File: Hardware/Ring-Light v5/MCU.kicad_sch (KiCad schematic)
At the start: 55 parts, among them J2 1017457000B11LF, J3 U.FL-R-SMT-1_80, J4 2002112100010C4LF, U37 CP2102N-A02-GQFN20R, U38 W25X40CLUXIG_TR, U39 CC2640R2FRGZR, Y1 32.768kHz, Y2 24MHz

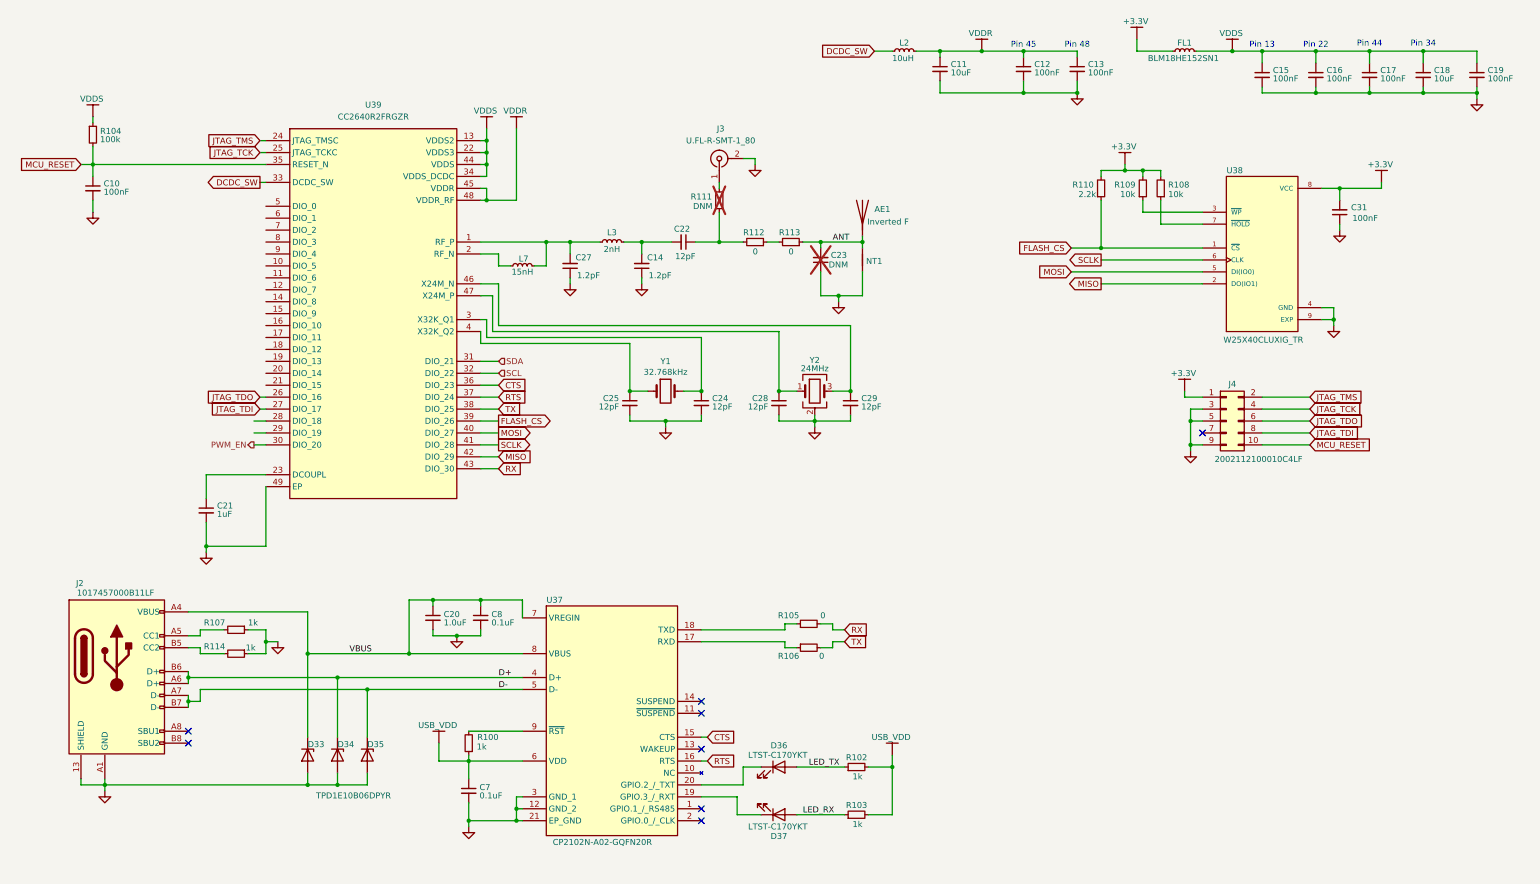
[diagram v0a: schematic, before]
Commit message: m
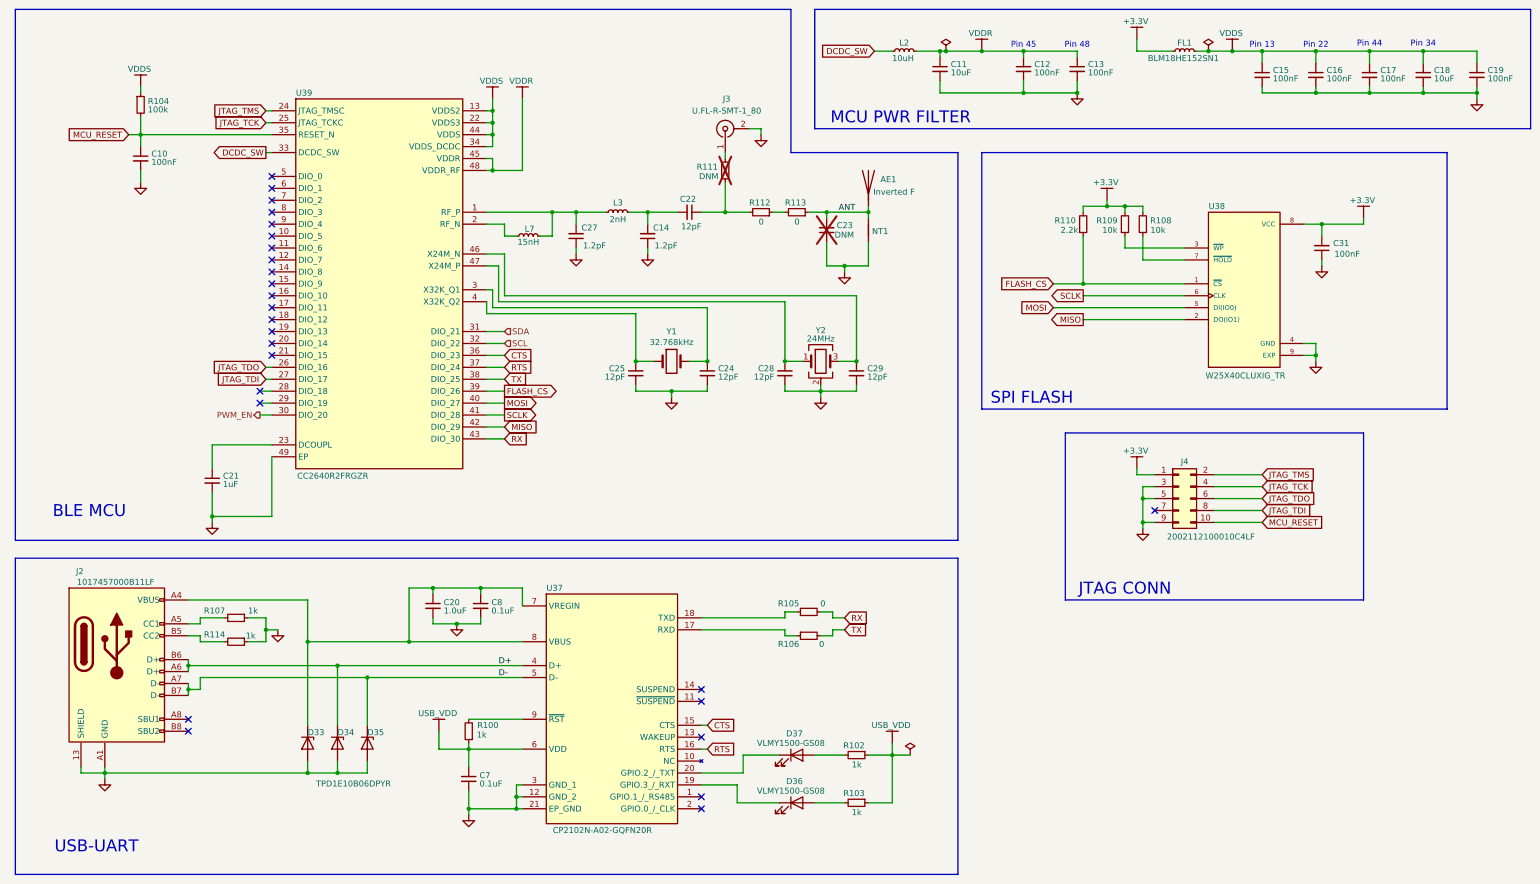
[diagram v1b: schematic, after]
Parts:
- removed J2: 1017457000B11LF, symbol Connector:USB_C_Receptacle
- removed J3: U.FL-R-SMT-1_80, Library:UFLRSMT180, symbol Connector:Conn_Coaxial
- added J2: 1017457000B11LF, Library:1017457000B11LF, symbol Library:1017457000B11LF
- added J3: U.FL-R-SMT-1_80, Library:UFLRSMT180, symbol Library:U.FL-R-SMT-1_80
- D33, D34, D35: footprint Library:TPD1E10B06DPYR -> Diode_SMD:D_SOD-523
- D36, D37: value LTST-C170YKT -> VLMY1500-GS08; footprint Diode_SMD:D_0402_1005Metric -> LED_SMD:LED_0402_1005Metric
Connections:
- net D+: now also J2.A6 (D+), J2.B6 (D+)
- net D-: now also J2.A7 (D-), J2.B7 (D-)
- net GND: now also J2.13 (SHIELD), J2.14 (SHIELD), J2.15 (SHIELD), J2.16 (SHIELD), J2.A1 (GND), J2.B1 (GND), J3.2 (Ext), J3.3 (Ext)
- net USB_VDD: now also R102.1, R103.1; no longer R102.2, R103.2
- net at C20.1, C8.1, D33.1 (K)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: now also J2.A4 (VBUS), J2.B4 (VBUS)
- net at C25.1, U39.4 (X32K_Q2): now also Y1.1; no longer Y1.2
- net at R114.2: now also J2.B5 (CC2)
- net at R107.2: now also J2.A5 (CC1)
- net at C24.1, U39.3 (X32K_Q1): now also Y1.2; no longer Y1.1
- net at R111.2: now also J3.1 (In)
- removed net LED_RX: D37.3 (A), D37.4 (A), R103.1
- removed net LED_TX: D36.3 (A), D36.4 (A), R102.1
- new net: D36.2 (A), R103.2
- new net: D36.1 (K), U37.19 (GPIO.3_/_RXT)
- new net: D37.1 (K), U37.20 (GPIO.2_/_TXT)
- new net: D37.2 (A), R102.2
- no-connect marks 8 -> 26
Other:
- note added: "BLE MCU"
- note added: "JTAG CONN"
- note added: "MCU PWR FILTER"
- note added: "SPI FLASH"
- note added: "USB-UART"
- moved on the sheet: AE1, C10, C14, C20, C21, C22, C23, C24, C25, C27, C28, C29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
